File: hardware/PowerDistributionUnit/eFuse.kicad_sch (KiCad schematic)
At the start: 27 parts, among them Q19 CSD18511Q5A, U4 AD5258, U5 TPS25983

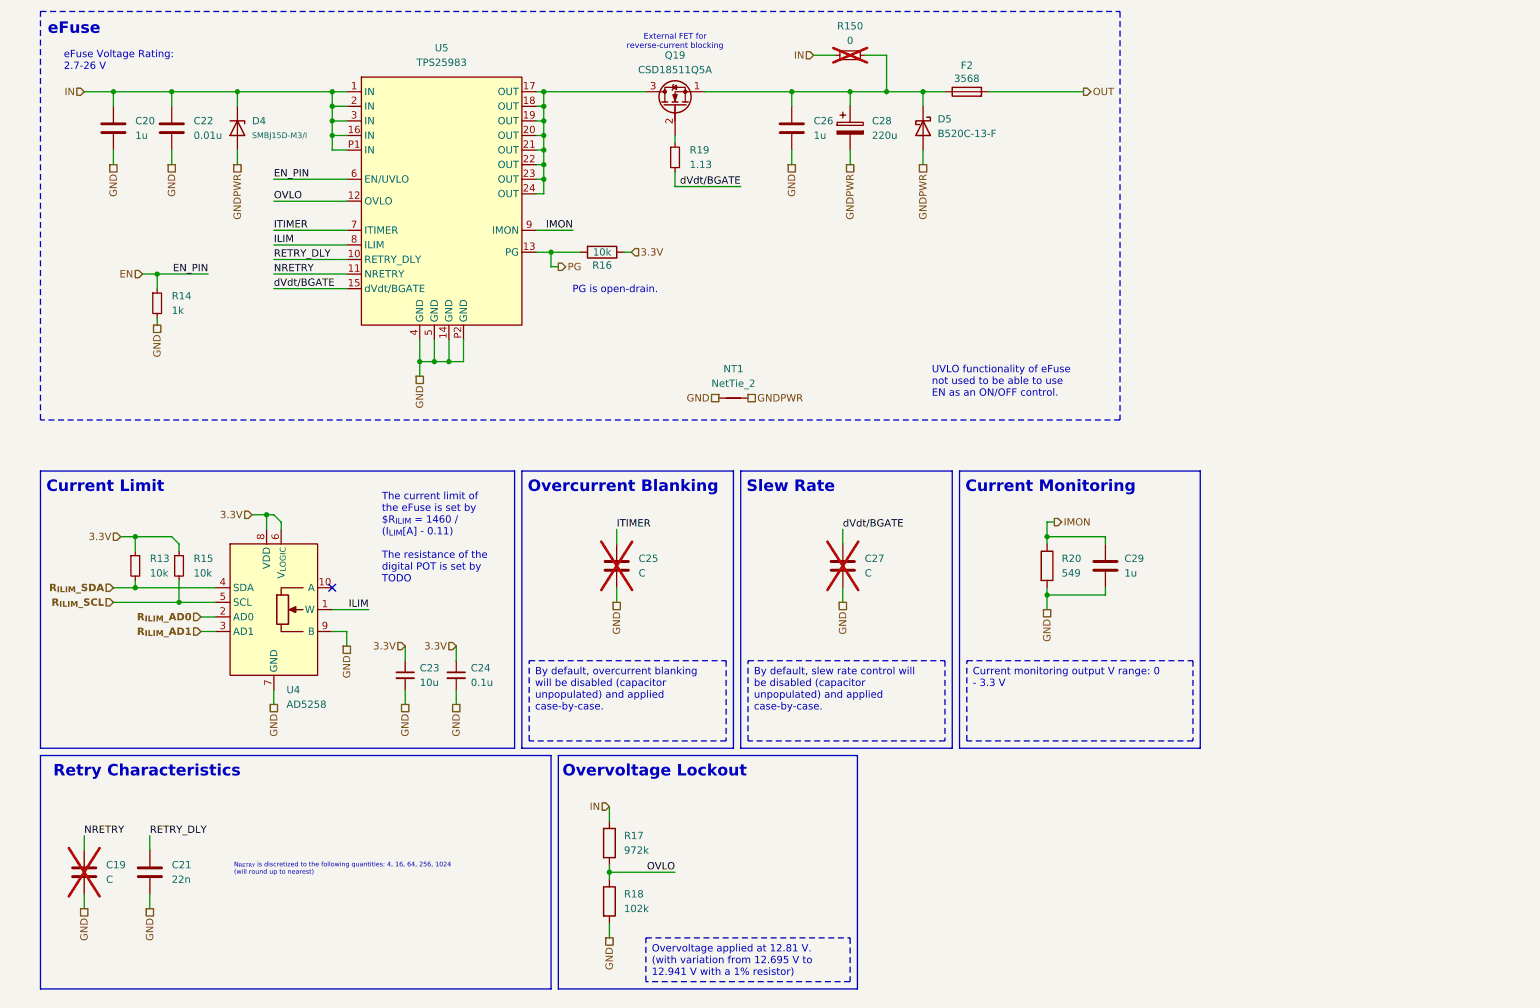
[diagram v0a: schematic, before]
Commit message: schematic updated
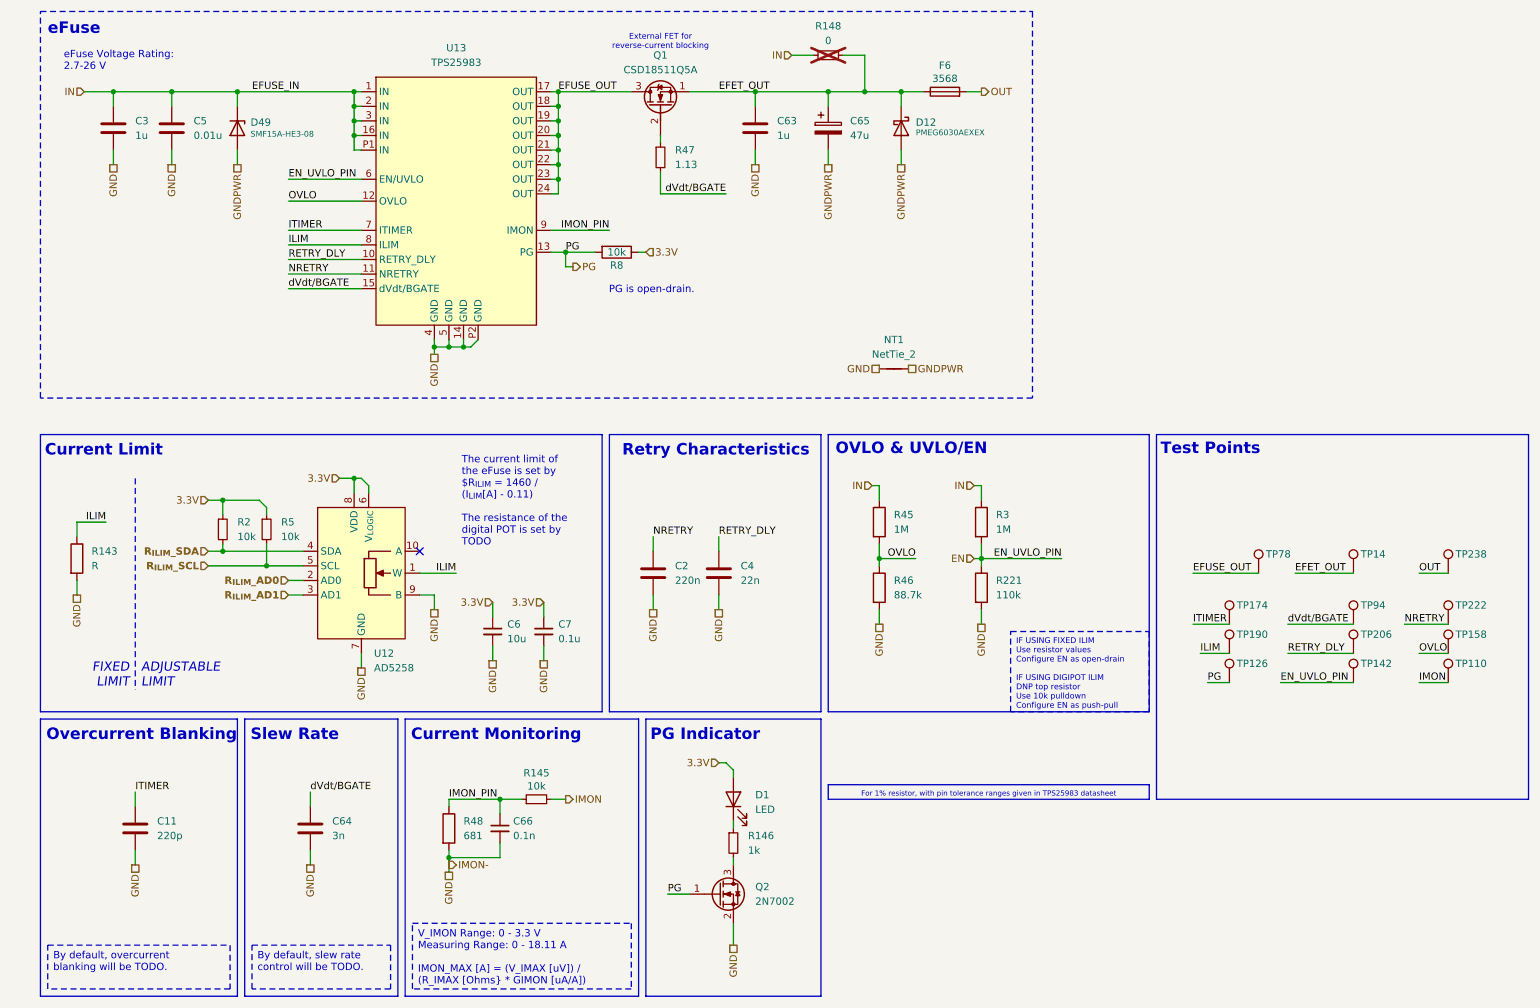
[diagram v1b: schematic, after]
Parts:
- removed D4: SMBJ15D-M3/I, Diode_SMD:D_SMB, symbol Device:D_Zener
- added D1: LED, LED_SMD:LED_0805_2012Metric, symbol Device:LED
- added D49: SMF15A-HE3-08, Diode_SMD:D_SMF, symbol Device:D_Zener
- added Q2: 2N7002, Package_TO_SOT_SMD:SOT-23, symbol Transistor_FET:Q_NMOS_GSD
- added R143: R, Resistor_SMD:R_0603_1608Metric, symbol Device:R
- added R145: 10k, Resistor_SMD:R_0603_1608Metric, symbol Device:R_Small
- added R146: 1k, Resistor_SMD:R_0603_1608Metric, symbol Device:R_Small
- added R221: 110k, Resistor_SMD:R_0603_1608Metric, symbol Device:R
- added TP110, TP126, TP14, TP142, TP158, TP174, TP190, TP206, TP222, TP78, TP94: TestPoint, TestPoint:TestPoint_Pad_D1.0mm, symbol Connector:TestPoint
- added TP238: TestPoint, Connector_PinHeader_2.54mm:PinHeader_1x01_P2.54mm_Vertical, symbol Connector:TestPoint
- C11: renamed from C25; value C -> 220p; footprint (none) -> Capacitor_SMD:C_0603_1608Metric; now fitted
- C2: renamed from C19; value C -> 220n; footprint (none) -> Capacitor_SMD:C_0603_1608Metric; now fitted
- C3: renamed from C20; footprint (none) -> Capacitor_SMD:C_0603_1608Metric
- C4: renamed from C21; footprint (none) -> Capacitor_SMD:C_0603_1608Metric
- C5: renamed from C22; footprint (none) -> Capacitor_SMD:C_0603_1608Metric
- C6: renamed from C23; footprint (none) -> Capacitor_SMD:C_0603_1608Metric
- C63: renamed from C26; footprint (none) -> Capacitor_SMD:C_0603_1608Metric
- C64: renamed from C27; value C -> 3n; footprint (none) -> Capacitor_SMD:C_0603_1608Metric; now fitted
- C65: renamed from C28; value 220u -> 47u; footprint Capacitor_SMD:CP_Elec_10x10.5 -> Capacitor_SMD:CP_Elec_6.3x4.9
- C66: renamed from C29; value 1u -> 0.1n; footprint (none) -> Capacitor_SMD:C_0603_1608Metric; symbol Device:C -> Device:C_Small
- C7: renamed from C24; footprint (none) -> Capacitor_SMD:C_0603_1608Metric
- D12: renamed from D5; value B520C-13-F -> PMEG6030AEXEX; footprint Diode_SMD:D_SMC -> PowerDistributionUnitLib:PMEG4030AEXEQX; Link (none) -> https://www.mouser.com/ProductDetail/Nexperia/PMEG6030AEXEX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
- NT1: footprint (none) -> NetTie:NetTie-2_SMD_Pad0.5mm
- R148: renamed from R150; footprint (none) -> Resistor_SMD:R_0603_1608Metric
- R2: renamed from R13; footprint (none) -> Resistor_SMD:R_0603_1608Metric
- R3: renamed from R14; value 1k -> 1M; footprint (none) -> Resistor_SMD:R_0603_1608Metric; symbol Device:R_Small -> Device:R
- R45: renamed from R17; value 972k -> 1M; footprint (none) -> Resistor_SMD:R_0603_1608Metric
- R46: renamed from R18; value 102k -> 88.7k; footprint (none) -> Resistor_SMD:R_0603_1608Metric
- R47: renamed from R19; footprint (none) -> Resistor_SMD:R_0603_1608Metric
- R48: renamed from R20; value 549 -> 681; footprint (none) -> Resistor_SMD:R_0603_1608Metric
- R5: renamed from R15; footprint (none) -> Resistor_SMD:R_0603_1608Metric
- R8: renamed from R16; footprint (none) -> Resistor_SMD:R_0603_1608Metric
- renumbered F2 to F6, Q19 to Q1, U4 to U12, U5 to U13
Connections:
- net 3.3V: now also D1.2 (A)
- net EN: now also R3.2, R221.1, TP142.1; no longer R3.1
- net GND: now also Q2.2 (S), R143.2, R221.2; no longer R3.2
- net GNDPWR: now also D49.2 (A)
- net ILIM: now also R143.1, TP190.1
- net IMON: now also R145.2, TP110.1; no longer C66.1, R48.1, U13.9 (IMON)
- net IN: now also R3.1, D49.1 (K)
- net ITIMER: now also TP174.1
- net NRETRY: now also TP222.1
- net OUT: now also TP238.1
- net OVLO: now also TP158.1
- net PG: now also Q2.1 (G), TP126.1
- net RETRY_DLY: now also TP206.1
- net dVdt/BGATE: now also TP94.1
- net EFET_OUT: now reaches C63.1, C65.1, D12.1 (K), F6.1, Q1.1 (S), R148.2
- net EFET_OUT: now also TP14.1
- net EFUSE_OUT: now reaches Q1.3 (D), U13.17 (OUT), U13.18 (OUT), U13.19 (OUT), U13.20 (OUT), U13.21 (OUT), U13.22 (OUT), U13.23 (OUT), U13.24 (OUT)
- net EFUSE_OUT: now also TP78.1
- new net: D1.1 (K), R146.1
- new net: Q2.3 (D), R146.2
- new net IMON_PIN: C66.1, R145.1, R48.1, U13.9 (IMON)
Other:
- note added: "ADJUSTABLE LIMIT"
- note added: "FIXED LIMIT"
- note added: "OVLO & UVLO/EN"
- note added: "PG Indicator"
- note added: "Test Points"
- note removed: "Overvoltage Lockout"
- note removed: "UVLO functionality of eFuse not used to be able to use EN as an ON/OFF control."
- company: (none) -> Longhorn Racing Solar
- title: (none) -> eFuse Output X
- moved on the sheet: C4, C6, C63, C65, C66, C7, D12, F6, NT1, Q1, R148, R2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
